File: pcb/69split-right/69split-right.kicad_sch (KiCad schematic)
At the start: 0 parts

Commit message: I think schematic is done?
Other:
- title: (none) -> 69SPLIT KEYBOARD
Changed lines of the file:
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@@
 	(generator_version "9.0")
 	(paper "A4")
+	(title_block
+		(title "69SPLIT KEYBOARD")
+		(date "2025-06-11")
+	)
 	(arc
 		(start 103.505 97.79)

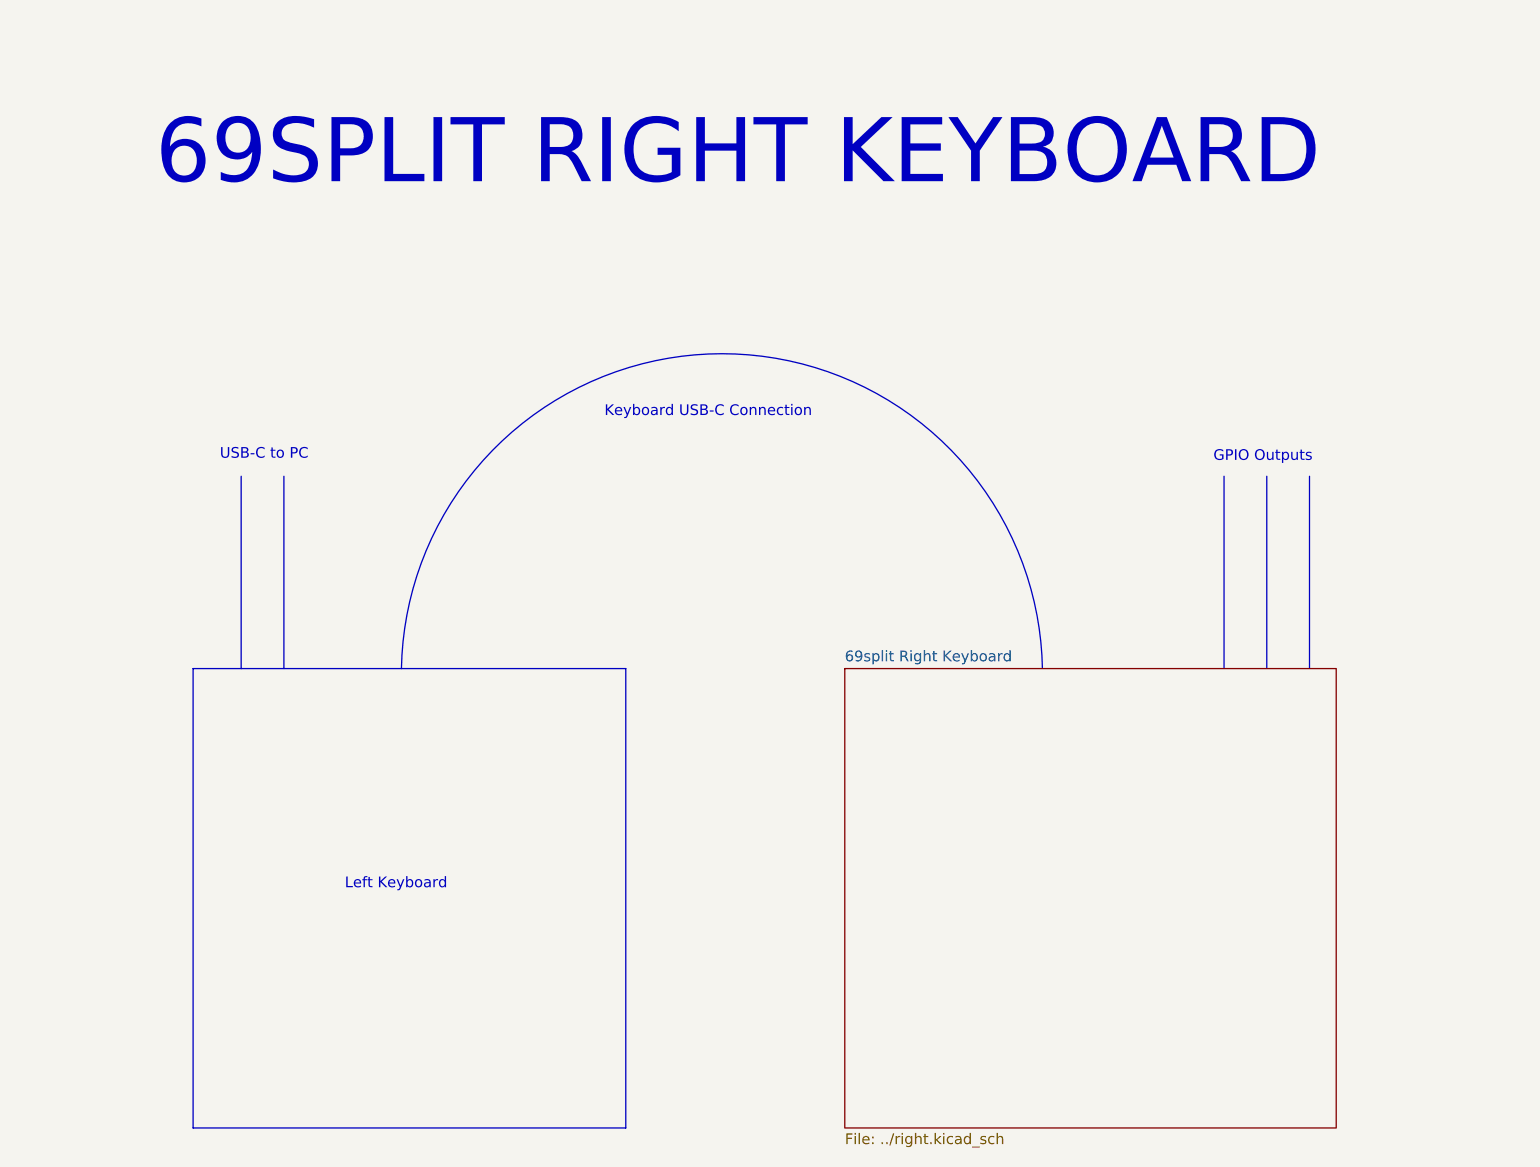
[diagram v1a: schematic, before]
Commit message: Moved things around so it's less confusing.
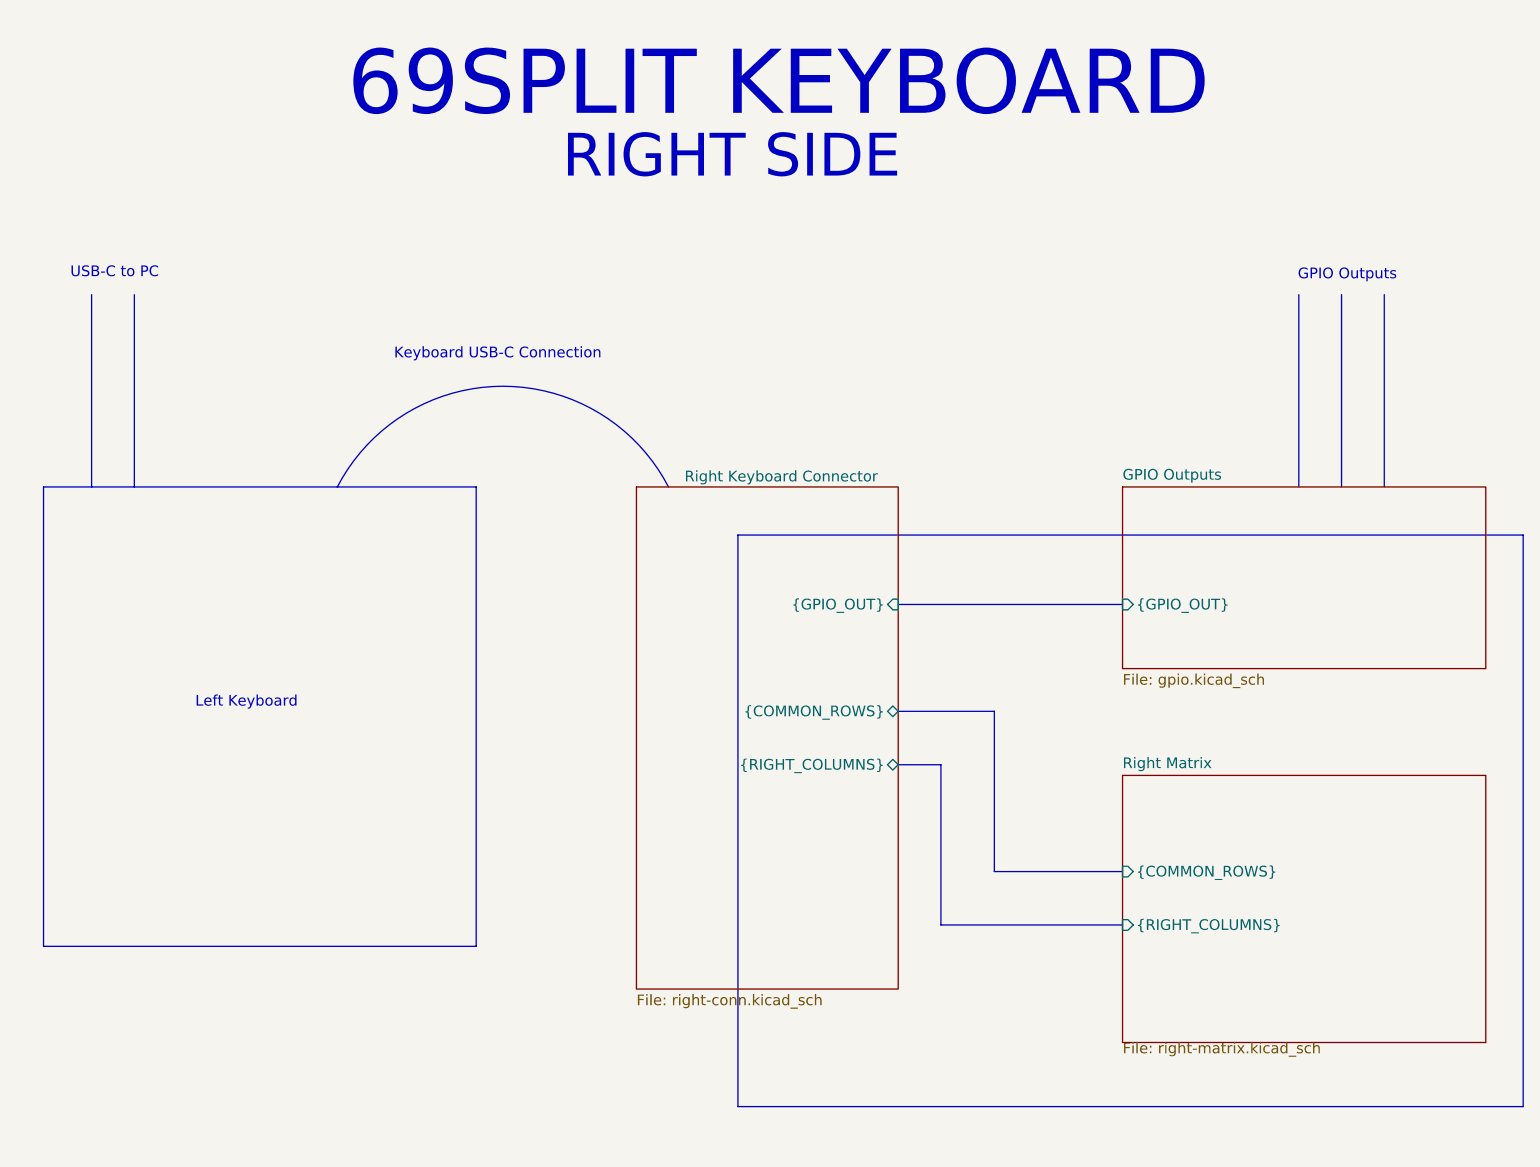
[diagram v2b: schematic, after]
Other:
- removed sheet 69split Right Keyboard
- added sheet GPIO Outputs (gpio.kicad_sch)
- added sheet Right Keyboard Connector (right-conn.kicad_sch)
- added sheet Right Matrix (right-matrix.kicad_sch)
- note added: "69SPLIT KEYBOARD"
- note added: "RIGHT SIDE"
- note removed: "69SPLIT RIGHT KEYBOARD"
